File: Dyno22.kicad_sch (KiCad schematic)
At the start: 49 parts, among them J2 Display, J3 Pwr Output, J4 BPM & Sensors, J5 Pwr Input, J7 UART, SW1 SW_DPST_x2, U1 TS2937CW50, U2 LM324, U3 Demux

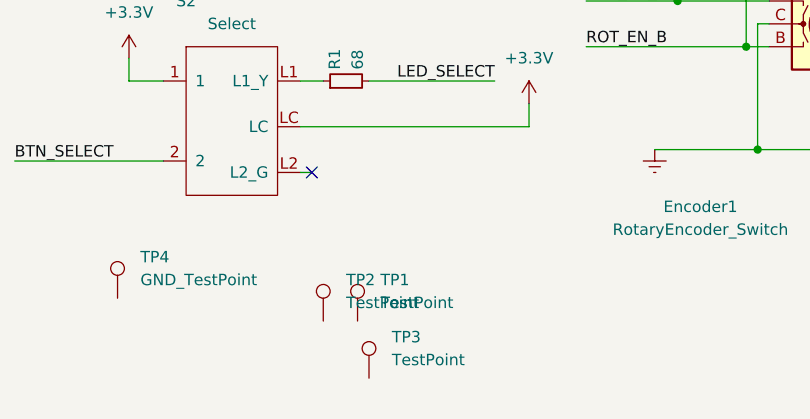
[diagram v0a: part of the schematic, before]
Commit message: schematic changes v2
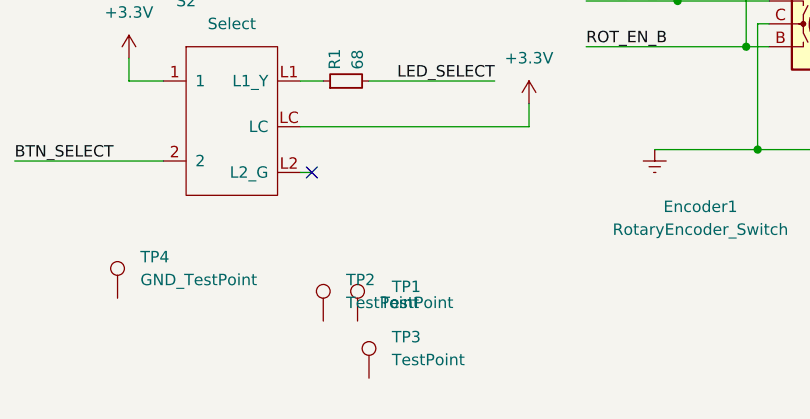
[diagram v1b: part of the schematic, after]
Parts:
- F1: footprint (none) -> Fuse:Fuse_1206_3216Metric
- SW1: footprint (none) -> Button_Switch_SMD:Nidec_Copal_SH-7040B
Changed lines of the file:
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@@
       (effects (font (size 1.27 1.27)))
     )
-    (property "Footprint" "" (at 115.57 48.26 0)
+    (property "Footprint" "Button_Switch_SMD:Nidec_Copal_SH-7040B" (at 115.57 48.26 0)
       (effects (font (size 1.27 1.27)) hide)
     )
@@
   )
   (symbol (lib_id "Connector:TestPoint") (at 69.85 186.69 0) (unit 1)
-    (in_bom yes) (on_board yes) (dnp no) (fields_autoplaced)
-    (property "Reference" "TP1" (at 72.39 182.118 0)
+    (in_bom yes) (on_board yes) (dnp no)
+    (property "Reference" "TP1" (at 73.66 182.88 0)
       (effects (font (size 1.27 1.27)) (justify left))
     )
@@
       (effects (font (size 1.27 1.27)))
     )
-    (property "Footprint" "" (at 124.46 50.038 90)
-      (effects (font (size 1.27 1.27)) hide)
-    )
-    (property "Datasheet" "~" (at 124.46 48.26 0)
-      (effects (font (size 1.27 1.27)) hide)
-    )
+    (property "Footprint" "Fuse:Fuse_1206_3216Metric" (at 124.46 50.038 90)
+      (effects (font (size 1.27 1.27)) hide)
+    )
+    (property "Datasheet" "https://www.digikey.ca/en/products/detail/eaton-electronics-division/CC12H4-5A-TR/2138898" (at 124.46 48.26 0)
+      (effects (font (size 1.27 1.27)) hide)
+    )
